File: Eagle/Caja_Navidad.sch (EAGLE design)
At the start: 24 parts, among them IC1 PIC16F877P

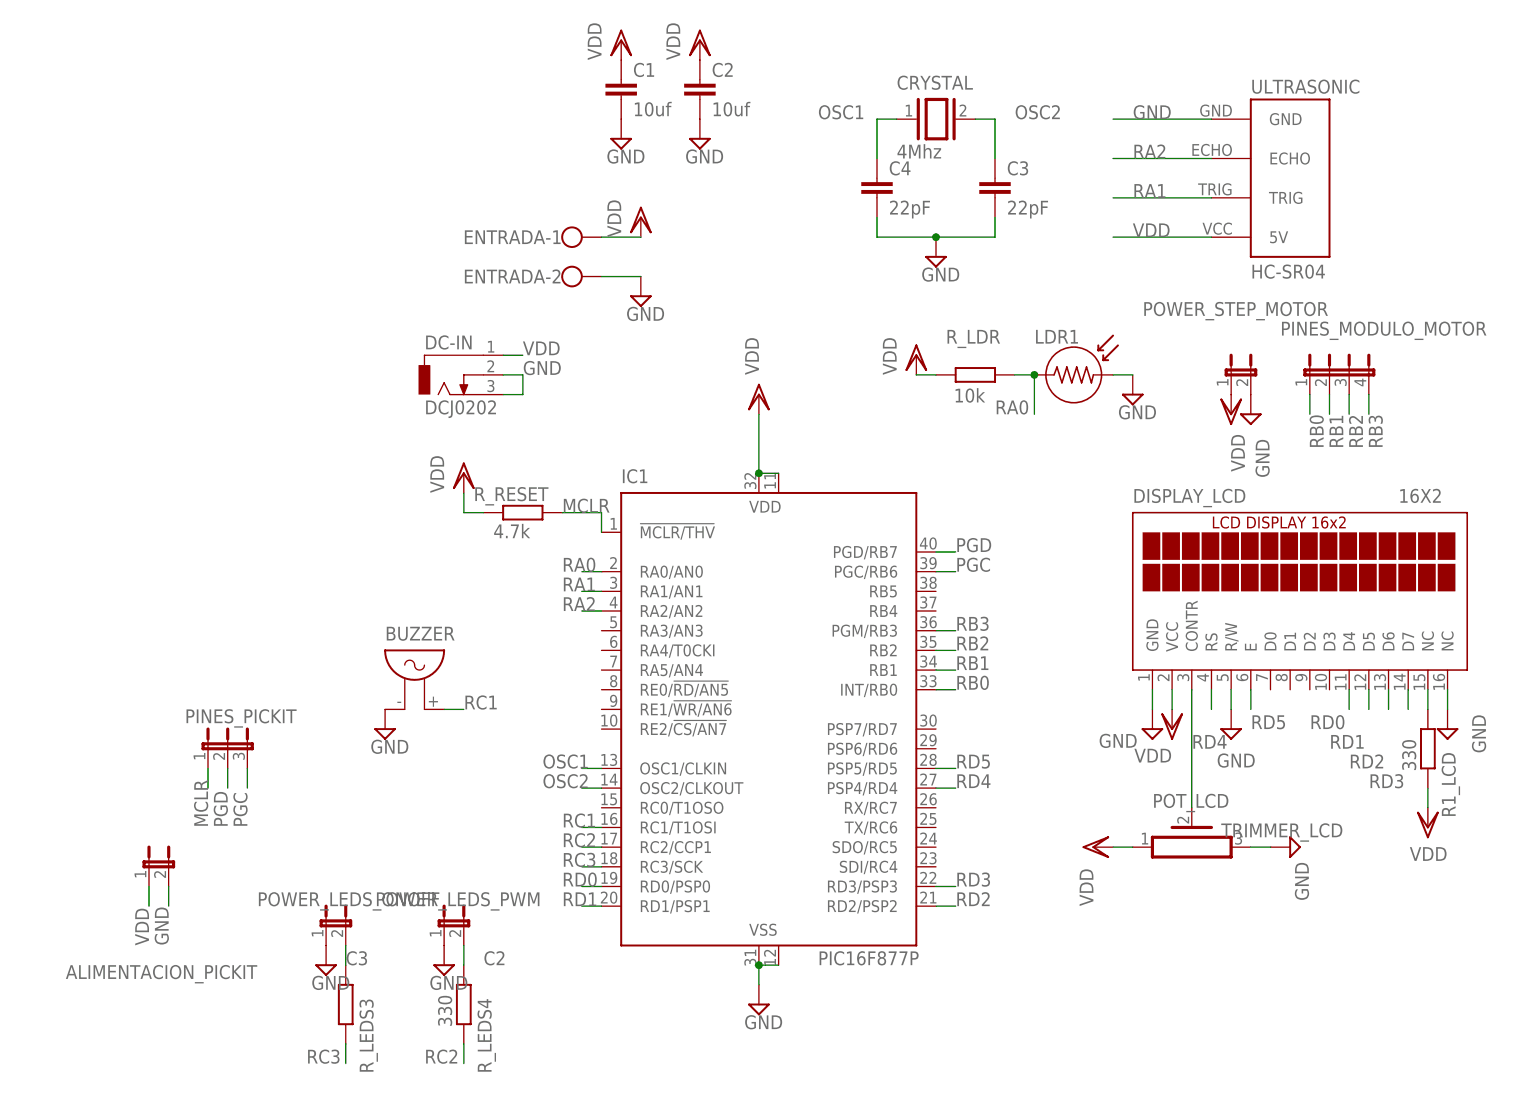
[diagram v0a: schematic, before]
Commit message: add Eagle Files v2
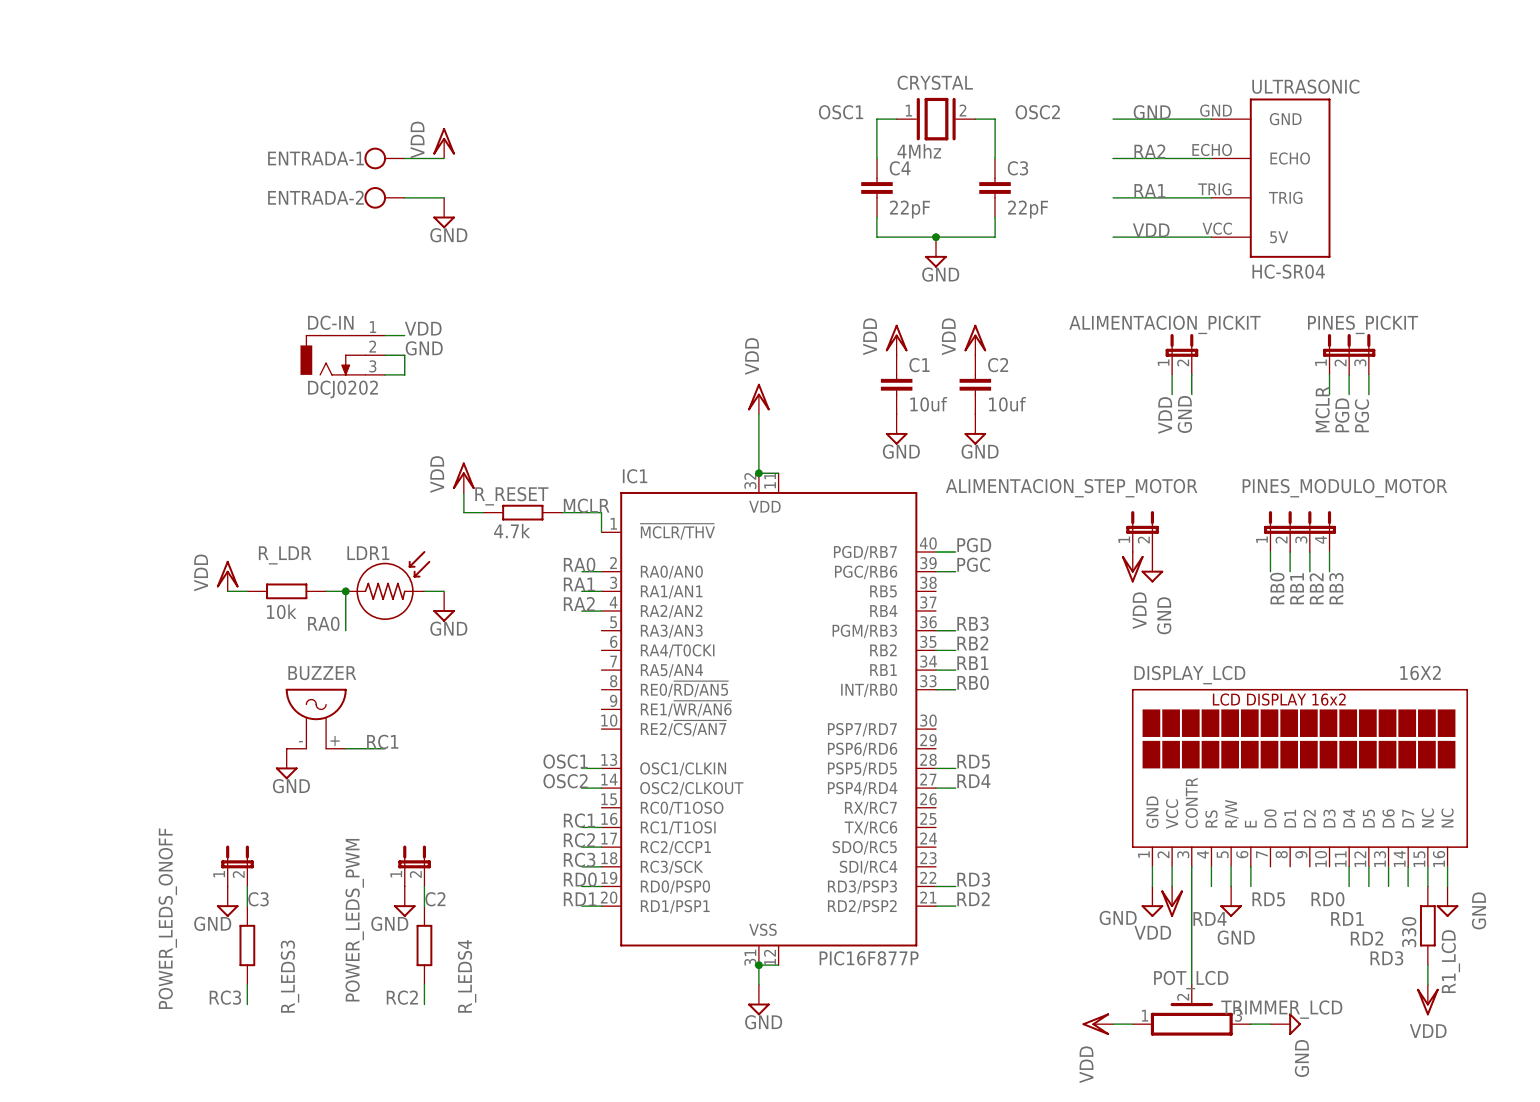
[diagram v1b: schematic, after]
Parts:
- removed POWER_STEP_MOTOR: (no value), jumper:JP1E
- added ALIMENTACION_STEP_MOTOR: (no value), jumper:JP1E
- R_LEDS4: value 330 -> (none)
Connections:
- net GND: now also ALIMENTACION_STEP_MOTOR.2; no longer POWER_STEP_MOTOR.2
- net VDD: now also ALIMENTACION_STEP_MOTOR.1; no longer POWER_STEP_MOTOR.1
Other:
- moved on the sheet: ALIMENTACION_PICKIT, BUZZER, C1, C2, DC-IN, DISPLAY_LCD, ENTRADA-1, ENTRADA-2, LDR1, PINES_MODULO_MOTOR, PINES_PICKIT, POWER_LEDS_ONOFF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
